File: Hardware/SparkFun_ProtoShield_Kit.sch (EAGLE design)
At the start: 29 parts

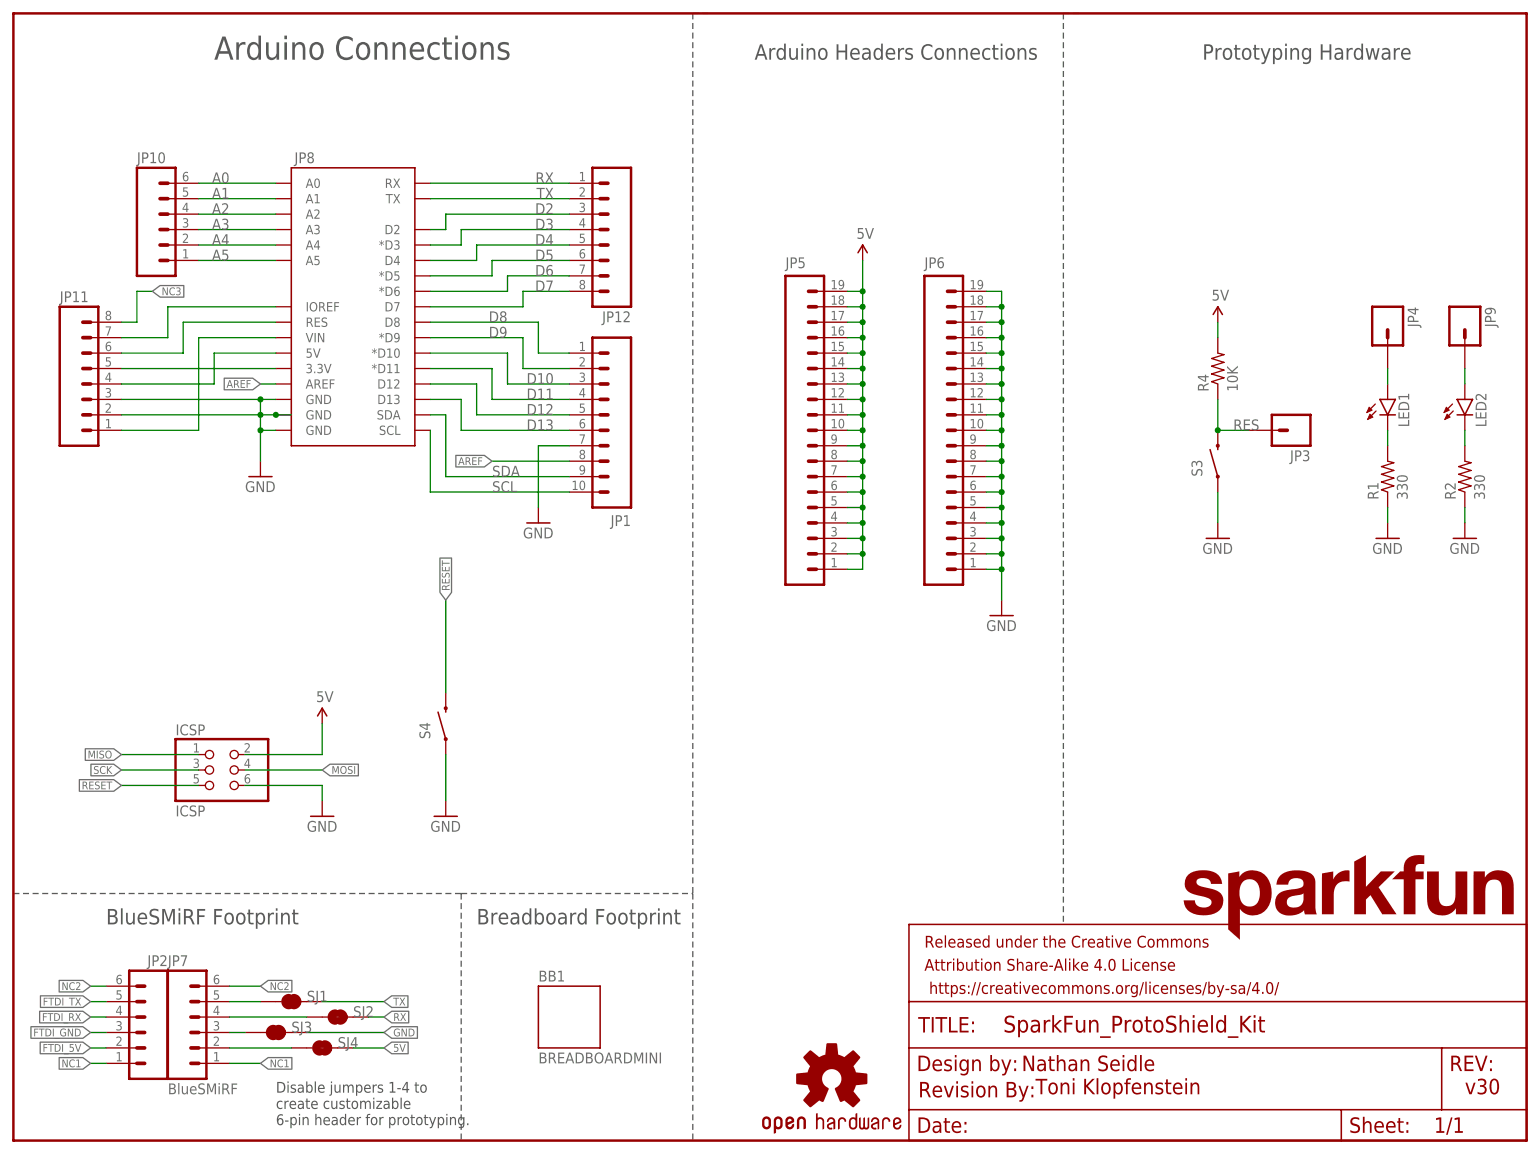
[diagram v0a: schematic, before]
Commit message: Updates from engineering review
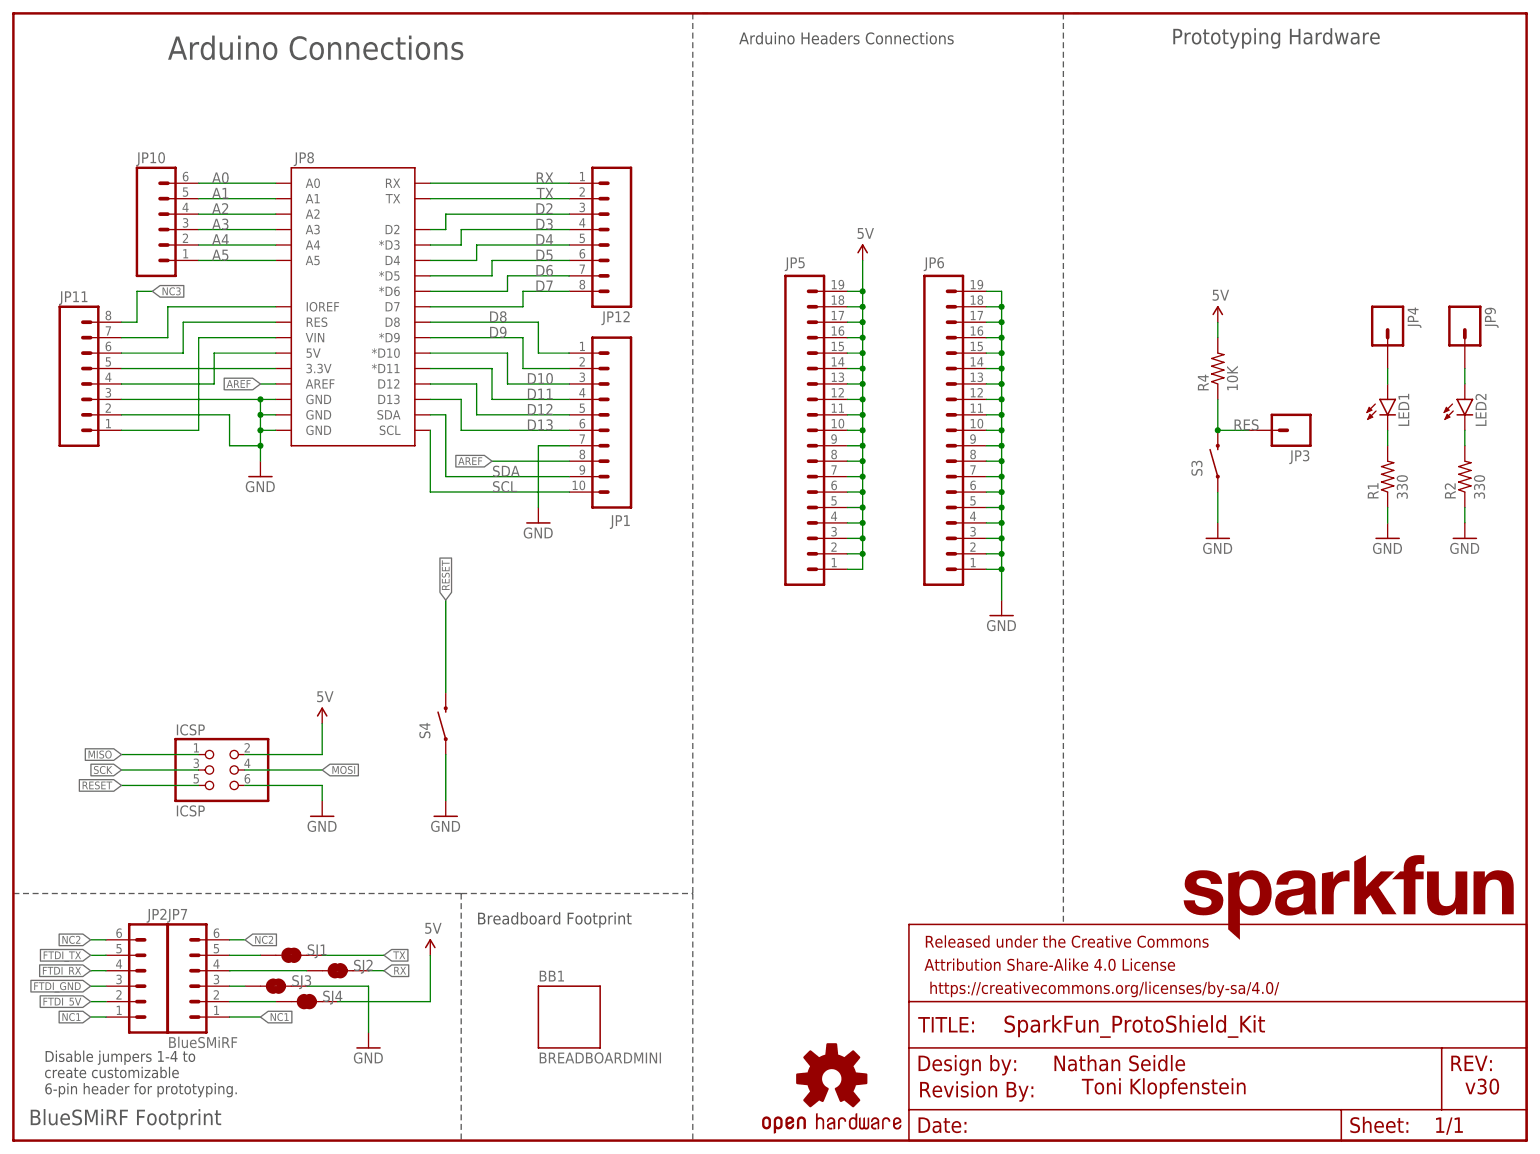
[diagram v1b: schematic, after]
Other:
- moved on the sheet: JP2, JP7, SJ1, SJ2, SJ3, SJ4
